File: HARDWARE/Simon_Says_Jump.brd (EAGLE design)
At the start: 64.8 x 99.1 mm, 62 parts, among them J1 RJ45, J10 B3, J11 LED_CTRLS, J12 5V, J13 5V, J14 B4, J15 B5, J16 B6, J17 B7, J19 12V, J2 RJ45, J20 RJ45, J21 12V, J22 12V, J3 RJ45, J4 RJ45, J6 5V, J8 B1, J9 B2, Q1 NPN, Q2 P-Channel MOSFET, Q3 NPN, Q4 P-Channel MOSFET, Q5 NPN, Q6 P-Channel MOSFET, Q7 NPN, Q8 P-Channel MOSFET, U1 5V Pro Mini, U2 LOGIC

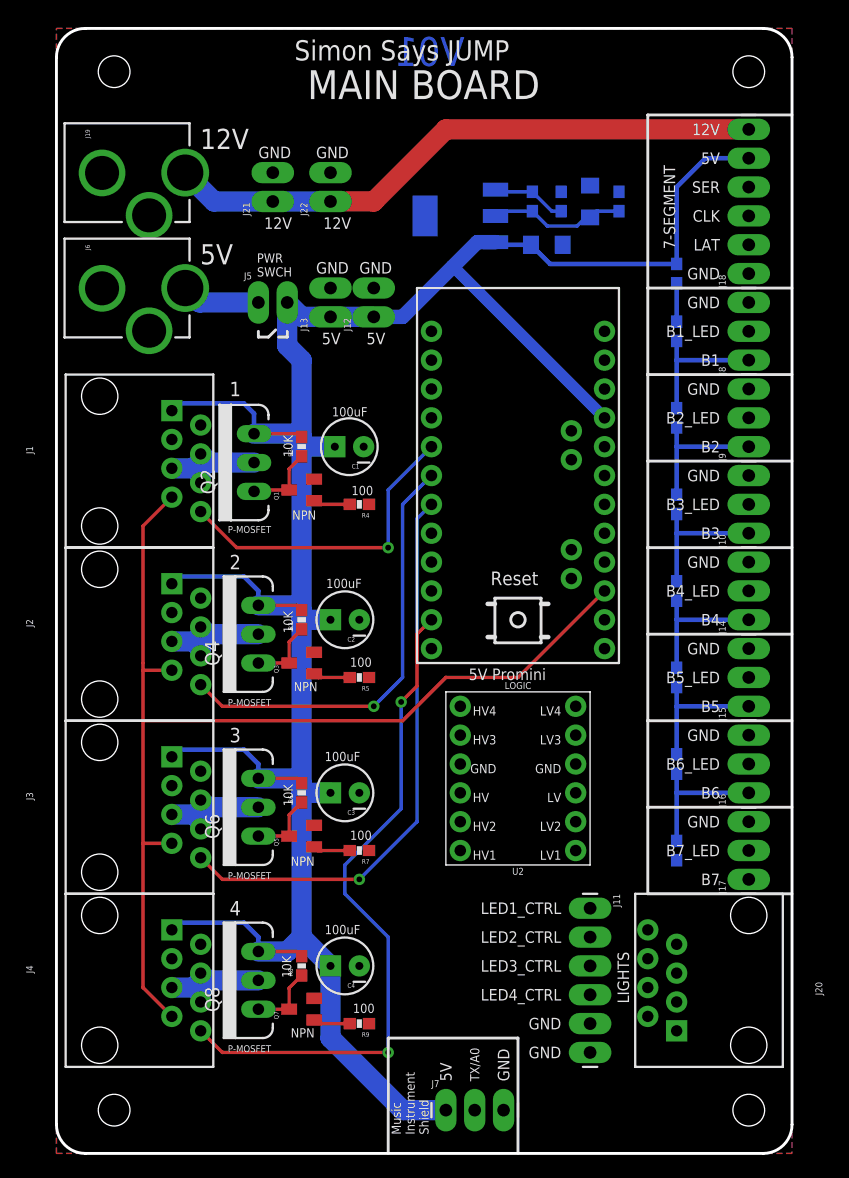
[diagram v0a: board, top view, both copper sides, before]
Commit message: more layout coming along
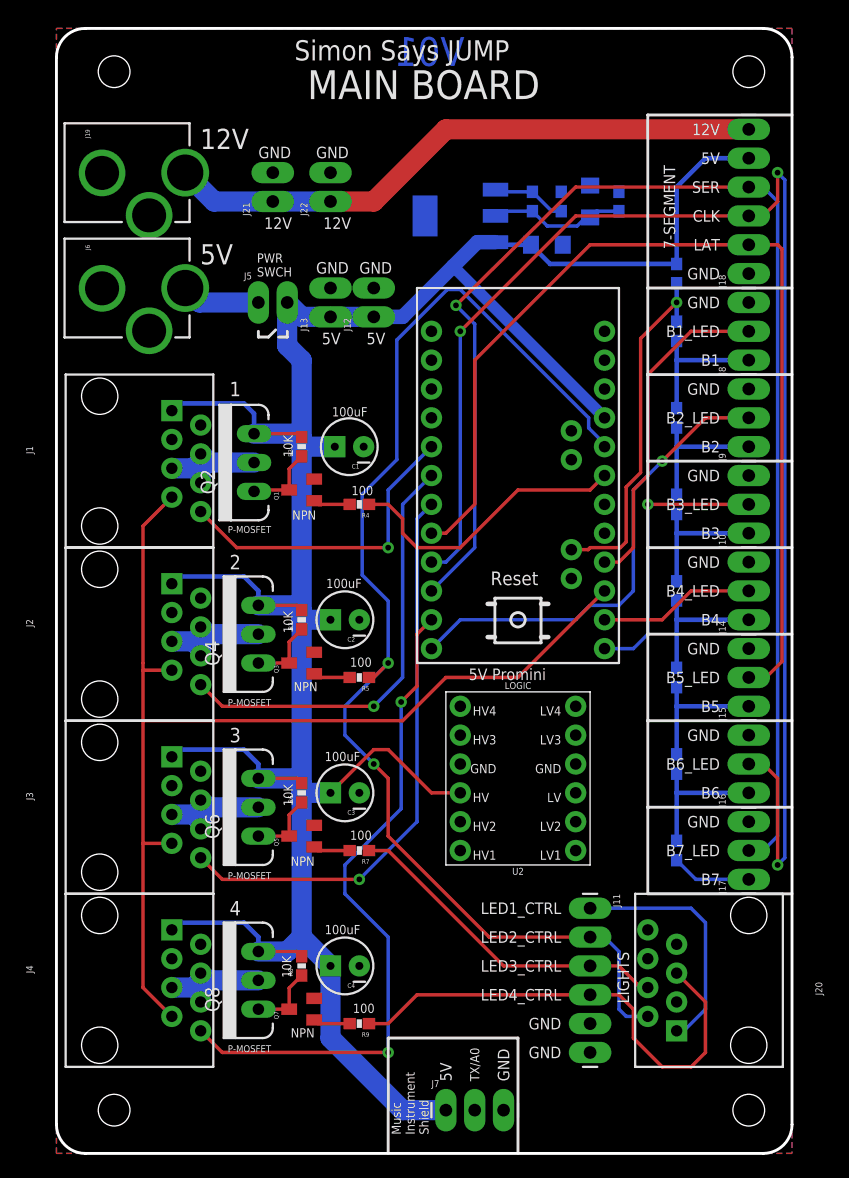
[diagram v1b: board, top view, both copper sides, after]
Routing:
- net CLK/B6_LED: track 0.00 -> 129.5 mm, vias 0 -> 3
- net SER/B7_LED: track 0.00 -> 119.5 mm, vias 0 -> 1
- net LED2_CTRL: track 0.00 -> 110.2 mm, vias 0 -> 2
- net LAT/B5_LED: track 0.00 -> 88.8 mm
- net LED1_CTRL: track 0.00 -> 47.3 mm
- net LED4_CTRL: track 0.00 -> 43.4 mm
- net B2_LED: track 0.00 -> 41.6 mm, vias 0 -> 1
- net LED3_CTRL: track 0.00 -> 29.5 mm
- net B1_LED: track 0.00 -> 29.3 mm
- net BUTTONS: track 3.38 -> 31.4 mm, vias 0 -> 1
- net B3_LED: track 0.00 -> 24.7 mm, vias 0 -> 1
- net 5V: track 230.1 -> 244.7 mm
- net B4_LED: track 0.00 -> 13.8 mm
- net N$17: track 0.00 -> 7.05 mm
